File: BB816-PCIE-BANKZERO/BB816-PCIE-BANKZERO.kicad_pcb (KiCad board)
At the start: 4 copper layers, 167.6 x 111.2 mm, 23 parts, among them J1 BB816_BreakoutA27_PCIex16, J1 Bypass, U1 AS7C256B-15PIN, U10 74HC138, U11 W65C51NxP, U12 W65C51NxP, U15 74HC32, U16 74HC138, U2 AS7C256B-15PIN, U23 74HC04, U3 AT28C256-15PU, U4 74HC138, U5 74HC148, U6 74HC125, U7 74HC283, U8 W65C22SxP, U9 74HC32

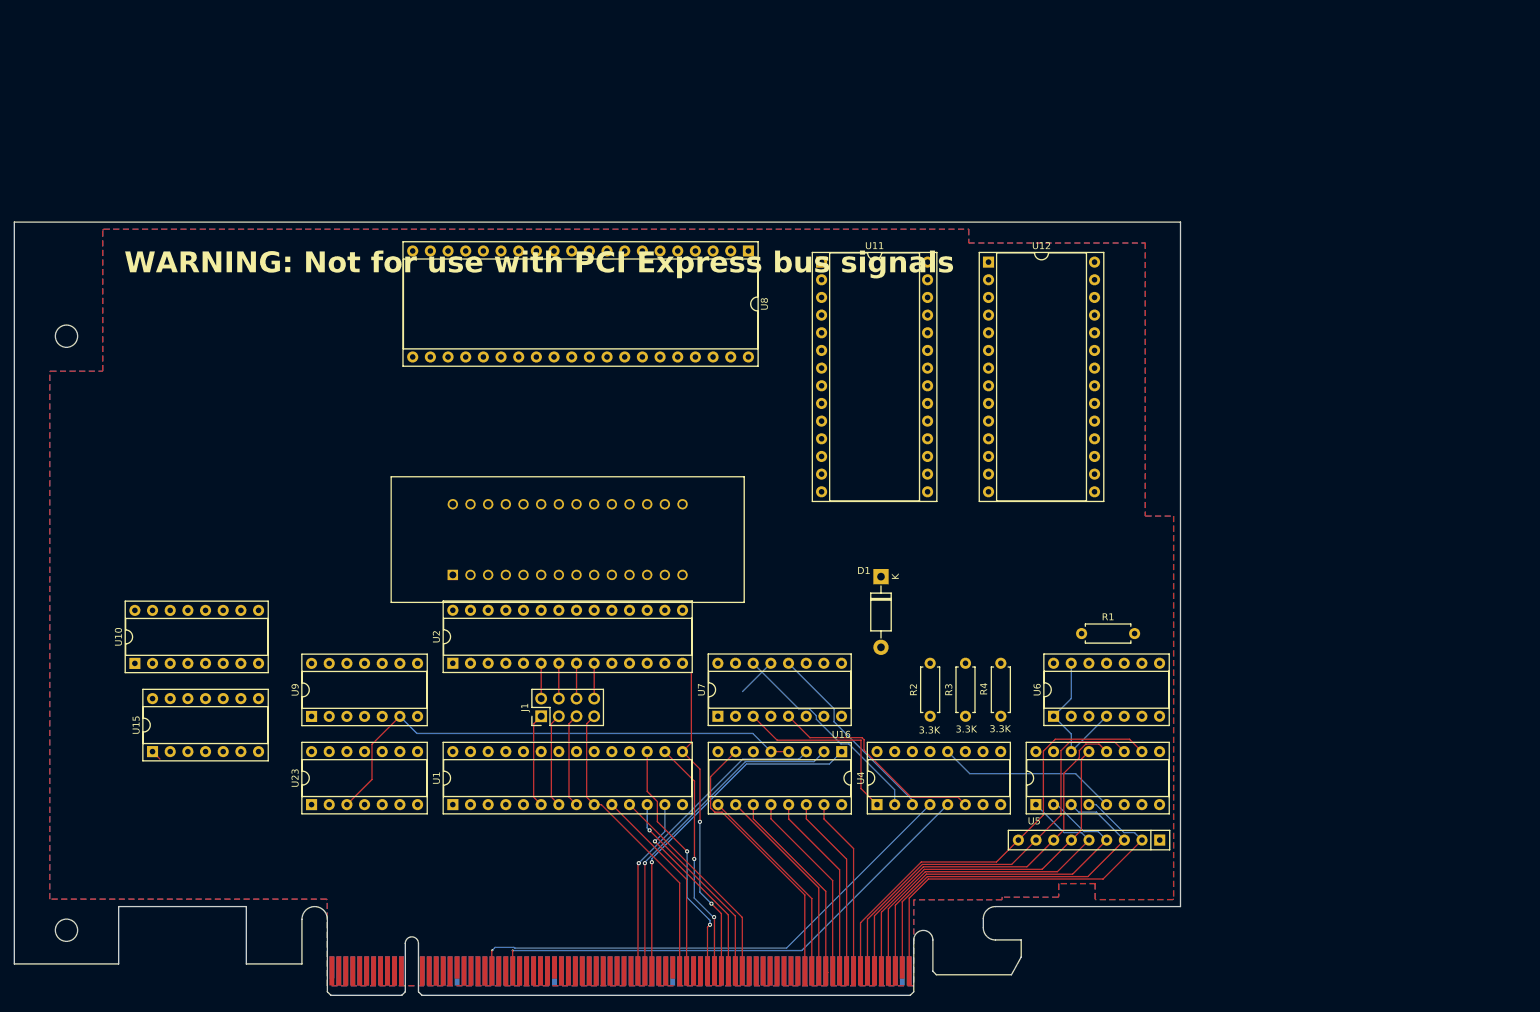
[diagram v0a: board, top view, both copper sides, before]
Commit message: VIA
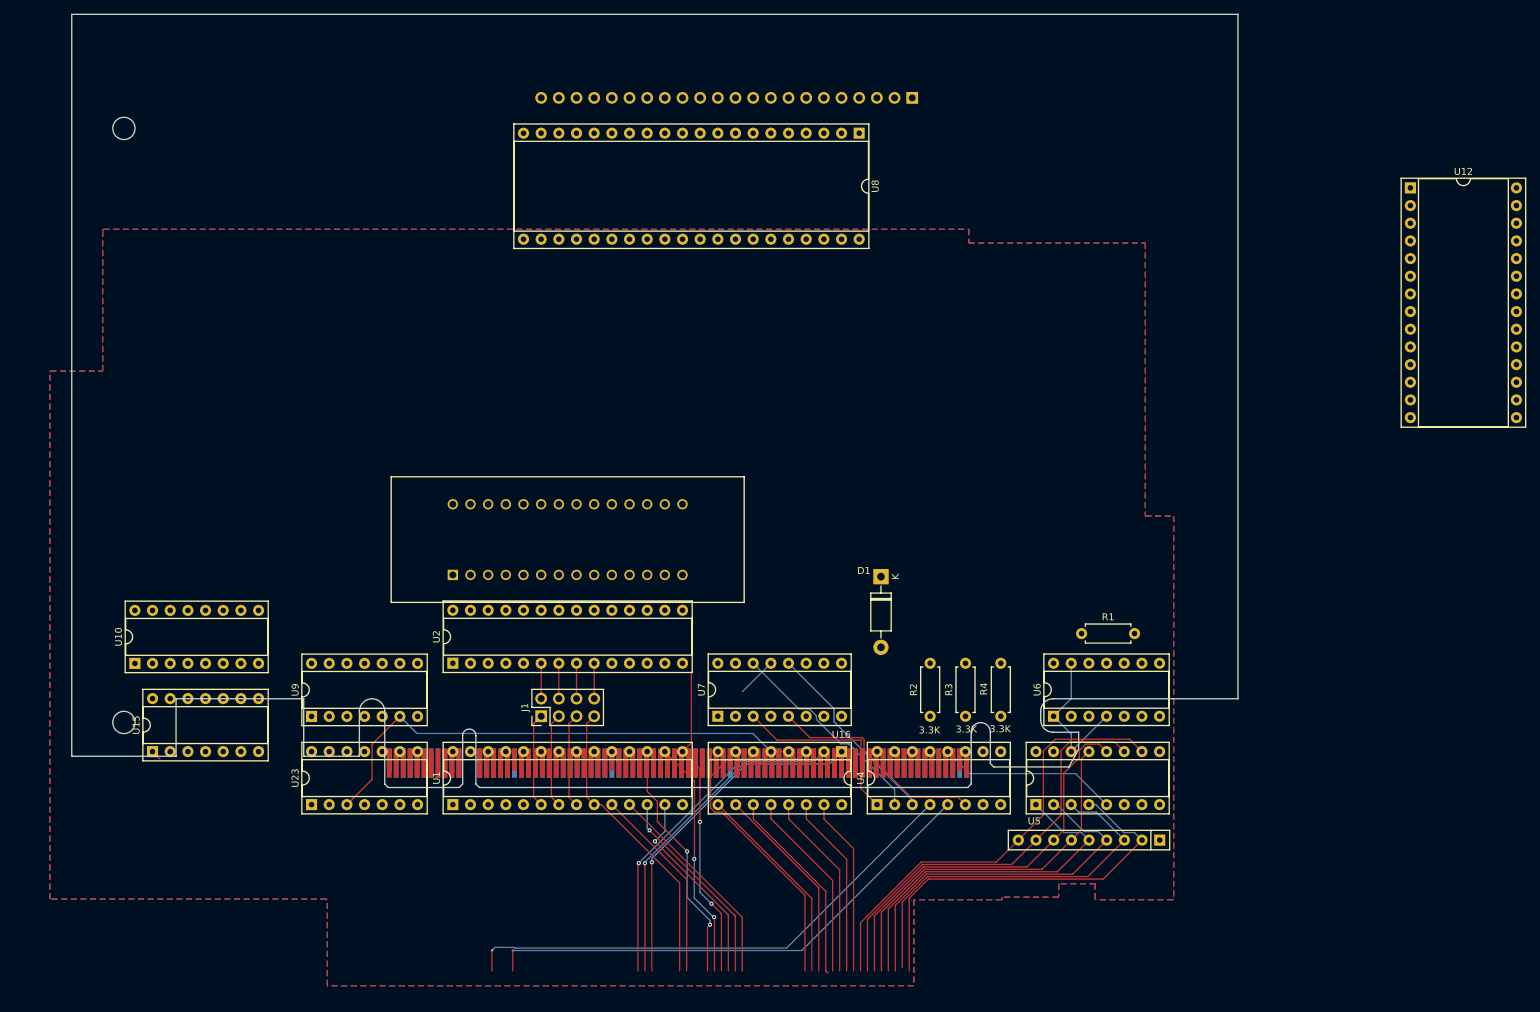
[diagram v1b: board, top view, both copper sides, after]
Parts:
- removed U11: W65C51NxP, Package_DIP:DIP-28_W15.24mm_Socket
- added J2: Conn_01x22_Pin, Connector_PinHeader_2.54mm:PinHeader_1x22_P2.54mm_Horizontal, B.Cu at (186.5, 24.0)
- moved U12 61.6 mm to (258.1, 36.9)
- moved J1 31.0 mm to (110.9, 123.1)
- moved U8 23.2 mm to (178.9, 29.1)
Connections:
- U8 pad 1: unconnected-(U8-VSS-Pad1) -> GND
- U8 pad 10: unconnected-(U8-PB0-Pad10) -> Net-(J2-Pin_13)
- U8 pad 11: unconnected-(U8-PB1-Pad11) -> Net-(J2-Pin_14)
- U8 pad 12: unconnected-(U8-PB2-Pad12) -> Net-(J2-Pin_15)
- U8 pad 13: unconnected-(U8-PB3-Pad13) -> Net-(J2-Pin_16)
- U8 pad 14: unconnected-(U8-PB4-Pad14) -> Net-(J2-Pin_17)
- U8 pad 15: unconnected-(U8-PB5-Pad15) -> Net-(J2-Pin_18)
- U8 pad 16: unconnected-(U8-PB6-Pad16) -> Net-(J2-Pin_19)
- U8 pad 17: unconnected-(U8-PB7-Pad17) -> Net-(J2-Pin_20)
- U8 pad 18: unconnected-(U8-CB1-Pad18) -> Net-(J2-Pin_21)
- U8 pad 19: unconnected-(U8-CB2-Pad19) -> Net-(J2-Pin_22)
- U8 pad 2: unconnected-(U8-PA0-Pad2) -> Net-(J2-Pin_3)
- U8 pad 20: unconnected-(U8-VCC-Pad20) -> VCC
- U8 pad 21: unconnected-(U8-~{IRQ}-Pad21) -> /~{IRQ0}
- U8 pad 22: unconnected-(U8-R/~{W}-Pad22) -> /~{RAM0_WE}
- U8 pad 23: unconnected-(U8-~{CS2}-Pad23) -> /~{IOCS0}
- U8 pad 24: unconnected-(U8-CS1-Pad24) -> VCC
- U8 pad 26: unconnected-(U8-D7-Pad26) -> /D7
- U8 pad 27: unconnected-(U8-D6-Pad27) -> /D6
- U8 pad 28: unconnected-(U8-D5-Pad28) -> /D5
- U8 pad 29: unconnected-(U8-D4-Pad29) -> /D4
- U8 pad 3: unconnected-(U8-PA1-Pad3) -> Net-(J2-Pin_4)
- U8 pad 30: unconnected-(U8-D3-Pad30) -> /D3
- U8 pad 31: unconnected-(U8-D2-Pad31) -> /D2
- U8 pad 32: unconnected-(U8-D1-Pad32) -> /D1
- U8 pad 33: unconnected-(U8-D0-Pad33) -> /D0
- U8 pad 35: unconnected-(U8-RS3-Pad35) -> /A3
- U8 pad 36: unconnected-(U8-RS2-Pad36) -> /A2
- U8 pad 37: unconnected-(U8-RS1-Pad37) -> /A1
- U8 pad 38: unconnected-(U8-RS0-Pad38) -> /A0
- U8 pad 39: unconnected-(U8-CA2-Pad39) -> Net-(J2-Pin_12)
- U8 pad 4: unconnected-(U8-PA2-Pad4) -> Net-(J2-Pin_5)
- U8 pad 40: unconnected-(U8-CA1-Pad40) -> Net-(J2-Pin_11)
- U8 pad 5: unconnected-(U8-PA3-Pad5) -> Net-(J2-Pin_6)
- U8 pad 6: unconnected-(U8-PA4-Pad6) -> Net-(J2-Pin_7)
- U8 pad 7: unconnected-(U8-PA5-Pad7) -> Net-(J2-Pin_8)
- U8 pad 8: unconnected-(U8-PA6-Pad8) -> Net-(J2-Pin_9)
- U8 pad 9: unconnected-(U8-PA7-Pad9) -> Net-(J2-Pin_10)
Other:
- board size 167.6 x 111.2 mm -> 167.6 x 111.1 mm
- board text removed: "WARNING: Not for use with PCI Express bus signals"

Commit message: Stuff
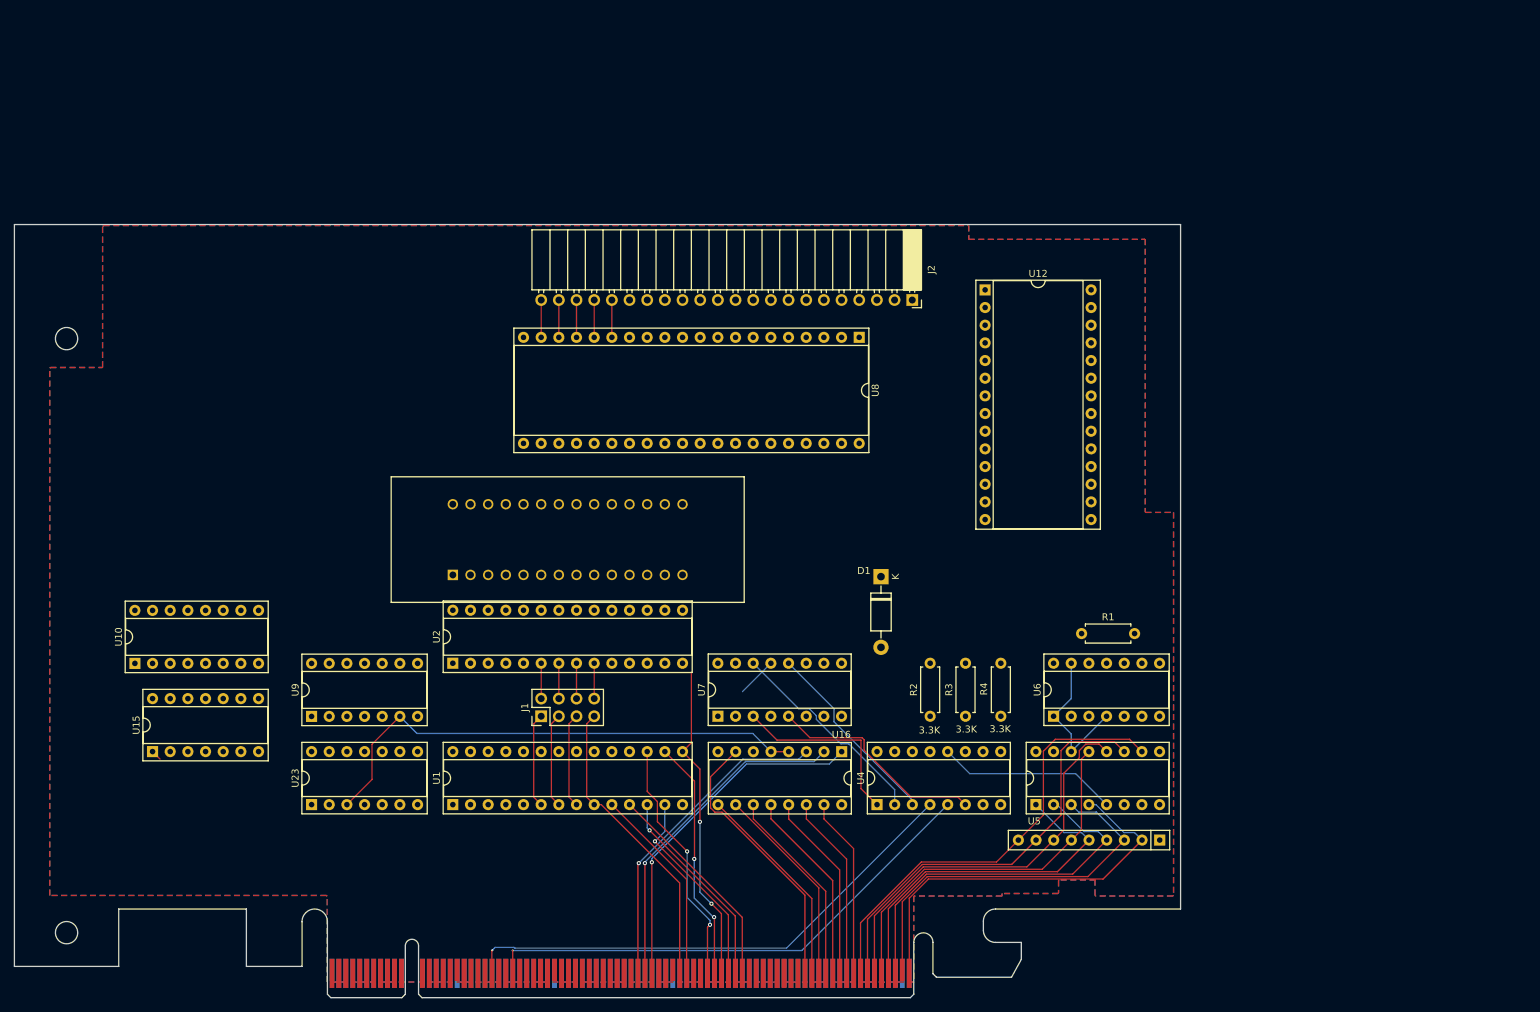
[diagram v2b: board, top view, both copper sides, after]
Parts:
- removed the J1 at (110.9, 123.1)
- added REF**: BUS_PCIexpress_x16, BB816-MATX-PCIE:PCIexpress_x16_HW_FH, F.Cu at (57.5, 42.2)
- J2: footprint Connector_PinHeader_2.54mm:PinHeader_1x22_P2.54mm_Horizontal -> Connector_PinSocket_2.54mm:PinSocket_1x22_P2.54mm_Horizontal; moved to F.Cu
- moved U12 62.9 mm to (197.0, 51.6)
- moved U8 29.4 mm to (178.9, 58.4)
- moved J2 29.1 mm to (186.5, 53.0), turned to -90 degrees
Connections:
- net Net-(J2-Pin_13) renamed /PB0
- net Net-(J2-Pin_14) renamed /PB1
- net Net-(J2-Pin_15) renamed /PB2
- net Net-(J2-Pin_16) renamed /PB3
- net Net-(J2-Pin_17) renamed /PB4
- net Net-(J2-Pin_18) renamed /PB5
- net Net-(J2-Pin_19) renamed /PB6
- net Net-(J2-Pin_20) renamed /PB7
- net Net-(J2-Pin_21) renamed /CB1
- net Net-(J2-Pin_22) renamed /CB2
- J2 pad 1: unconnected-(J2-Pin_1-Pad1) -> VCC
- J2 pad 10: Net-(J2-Pin_10) -> /PA5
- J2 pad 11: Net-(J2-Pin_11) -> /PA6
- J2 pad 12: Net-(J2-Pin_12) -> /PA7
- J2 pad 2: unconnected-(J2-Pin_2-Pad2) -> GND
- J2 pad 3: Net-(J2-Pin_3) -> /CA1
- J2 pad 4: Net-(J2-Pin_4) -> /CA2
- J2 pad 5: Net-(J2-Pin_5) -> /PA0
- J2 pad 6: Net-(J2-Pin_6) -> /PA1
- J2 pad 7: Net-(J2-Pin_7) -> /PA2
- J2 pad 8: Net-(J2-Pin_8) -> /PA3
- J2 pad 9: Net-(J2-Pin_9) -> /PA4
- U8 pad 2: Net-(J2-Pin_3) -> /PA0
- U8 pad 25: unconnected-(U8-ϕ2-Pad25) -> /CLK
- U8 pad 3: Net-(J2-Pin_4) -> /PA1
- U8 pad 39: Net-(J2-Pin_12) -> /CA2
- U8 pad 4: Net-(J2-Pin_5) -> /PA2
- U8 pad 40: Net-(J2-Pin_11) -> /CA1
- U8 pad 5: Net-(J2-Pin_6) -> /PA3
- U8 pad 6: Net-(J2-Pin_7) -> /PA4
- U8 pad 7: Net-(J2-Pin_8) -> /PA5
- U8 pad 8: Net-(J2-Pin_9) -> /PA6
- U8 pad 9: Net-(J2-Pin_10) -> /PA7
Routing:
- net /PB7: track 0.00 -> 5.37 mm
- net /PB6: track 0.00 -> 5.37 mm
- net /PB5: track 0.00 -> 5.37 mm
- net /CB2: track 0.00 -> 5.37 mm
- net /CB1: track 0.00 -> 5.37 mm
- added copper zone on B.Cu, net (none)
- added copper zone on F.Cu, net (none)
- added copper zone on In1.Cu, net (none)
- added copper zone on In2.Cu, net (none)
- removed copper zone on In1.Cu, net GND
- removed copper zone on In2.Cu, net GND
- removed copper zone on B.Cu, net VCC
- removed copper zone on F.Cu, net VCC
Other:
- board size 167.6 x 111.1 mm -> 167.7 x 111.1 mm
